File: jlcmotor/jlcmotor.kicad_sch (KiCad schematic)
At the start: 16 parts, among them J1 ScrewTerminal, U1 PinHeader8, U2 PinHeader8

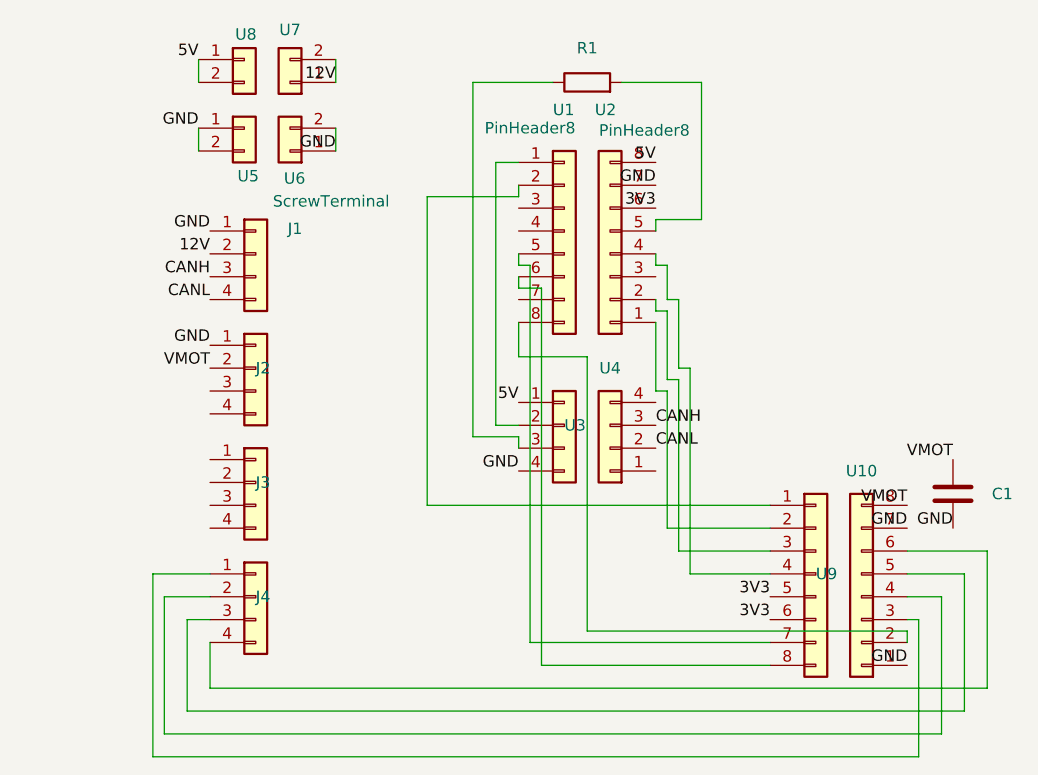
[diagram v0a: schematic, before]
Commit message: limit sw
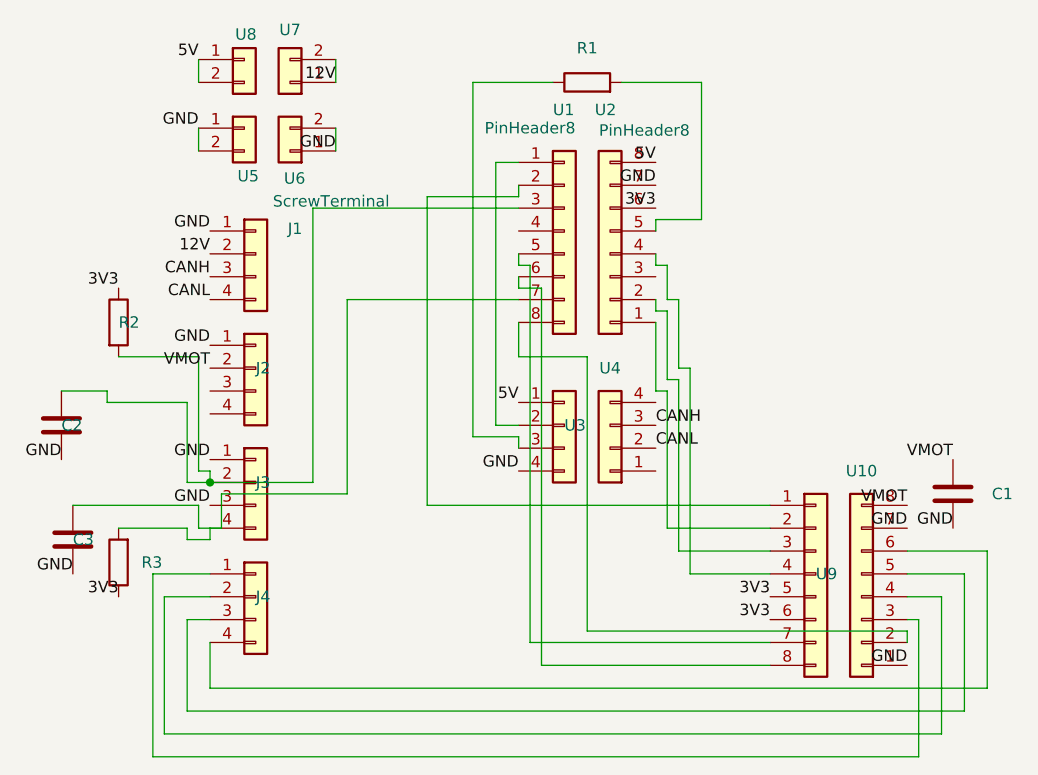
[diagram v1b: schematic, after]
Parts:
- added C2, C3: (no value), Capacitor_SMD:C_0603_1608Metric, symbol Device:C
- added R2, R3: (no value), Resistor_SMD:R_0603_1608Metric, symbol Device:R
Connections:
- net 3V3: now also R2.1, R3.1
- net GND: now also J3.1 (Pin_1), J3.3 (Pin_3), C2.2, C3.2
- net at J3.2 (Pin_2): now also U1.3 (Pin_3), C2.1, R2.2
- net at J3.4 (Pin_4): now also U1.7 (Pin_7), C3.1, R3.2
- net at J2.3 (Pin_3): no longer names the net of J2.3 (Pin_3)
- net at J2.3 (Pin_3): no longer J2.4 (Pin_4)
